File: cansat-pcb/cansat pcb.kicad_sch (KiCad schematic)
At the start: 19 parts, among them J1 Conn_01x03_Pin, J2 Conn_01x03_Pin, J3 Conn_01x03_Pin, Q1 2N3904, Q2 AO3400A, SW1 SW_DPDT_x2, U3 MPU6050

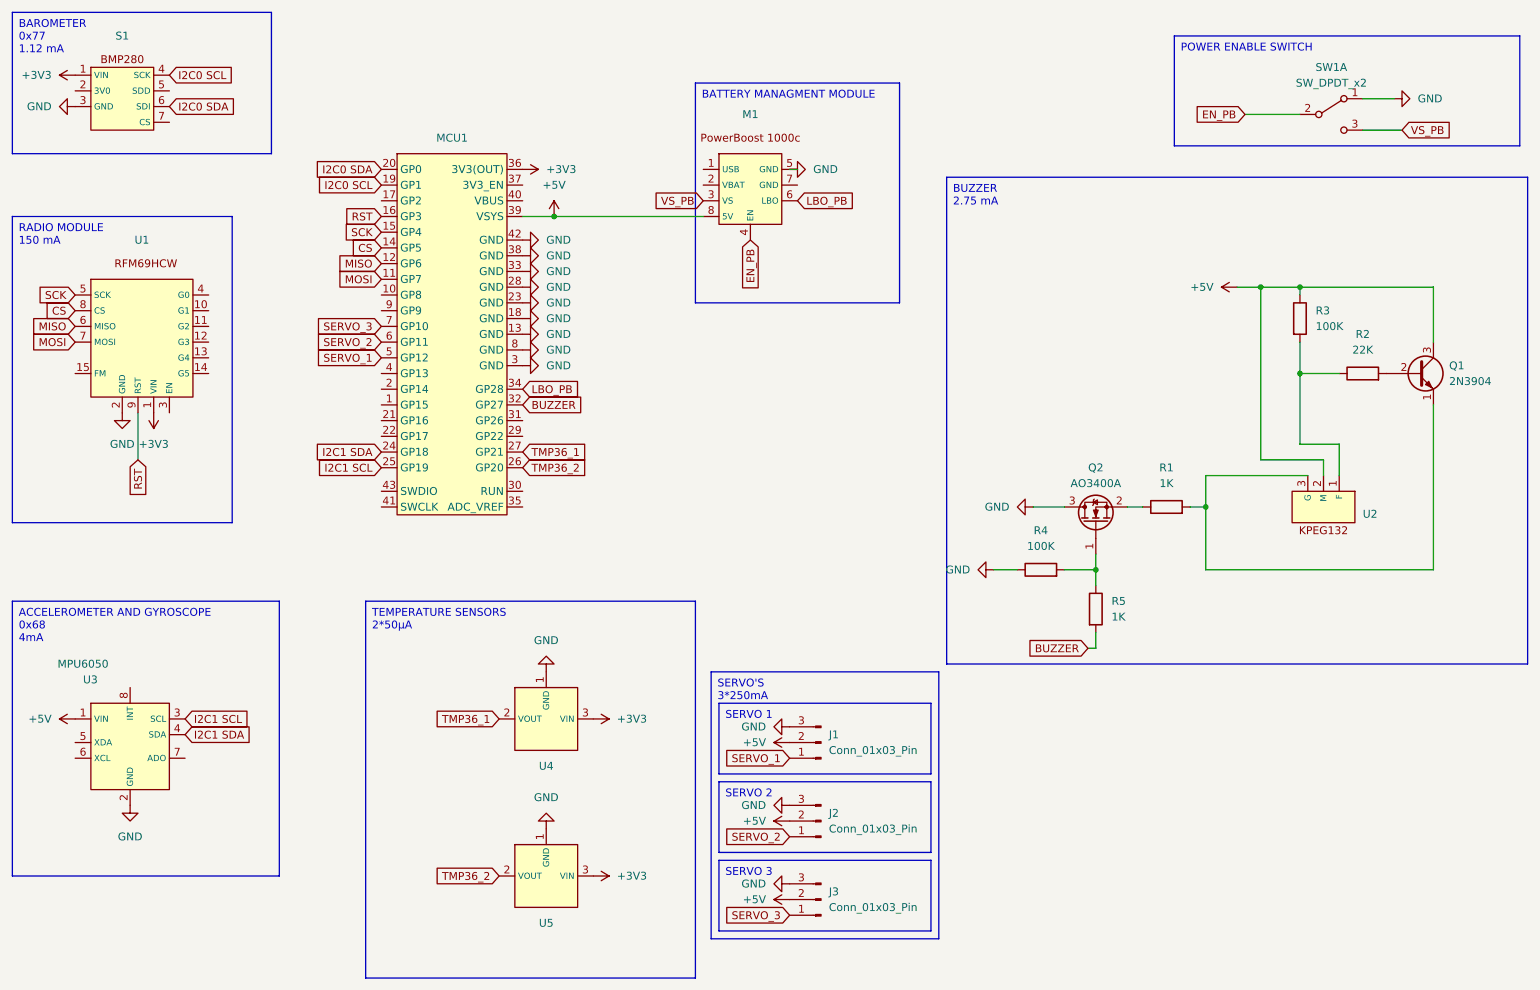
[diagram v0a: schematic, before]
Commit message: created MARKDOWN.md
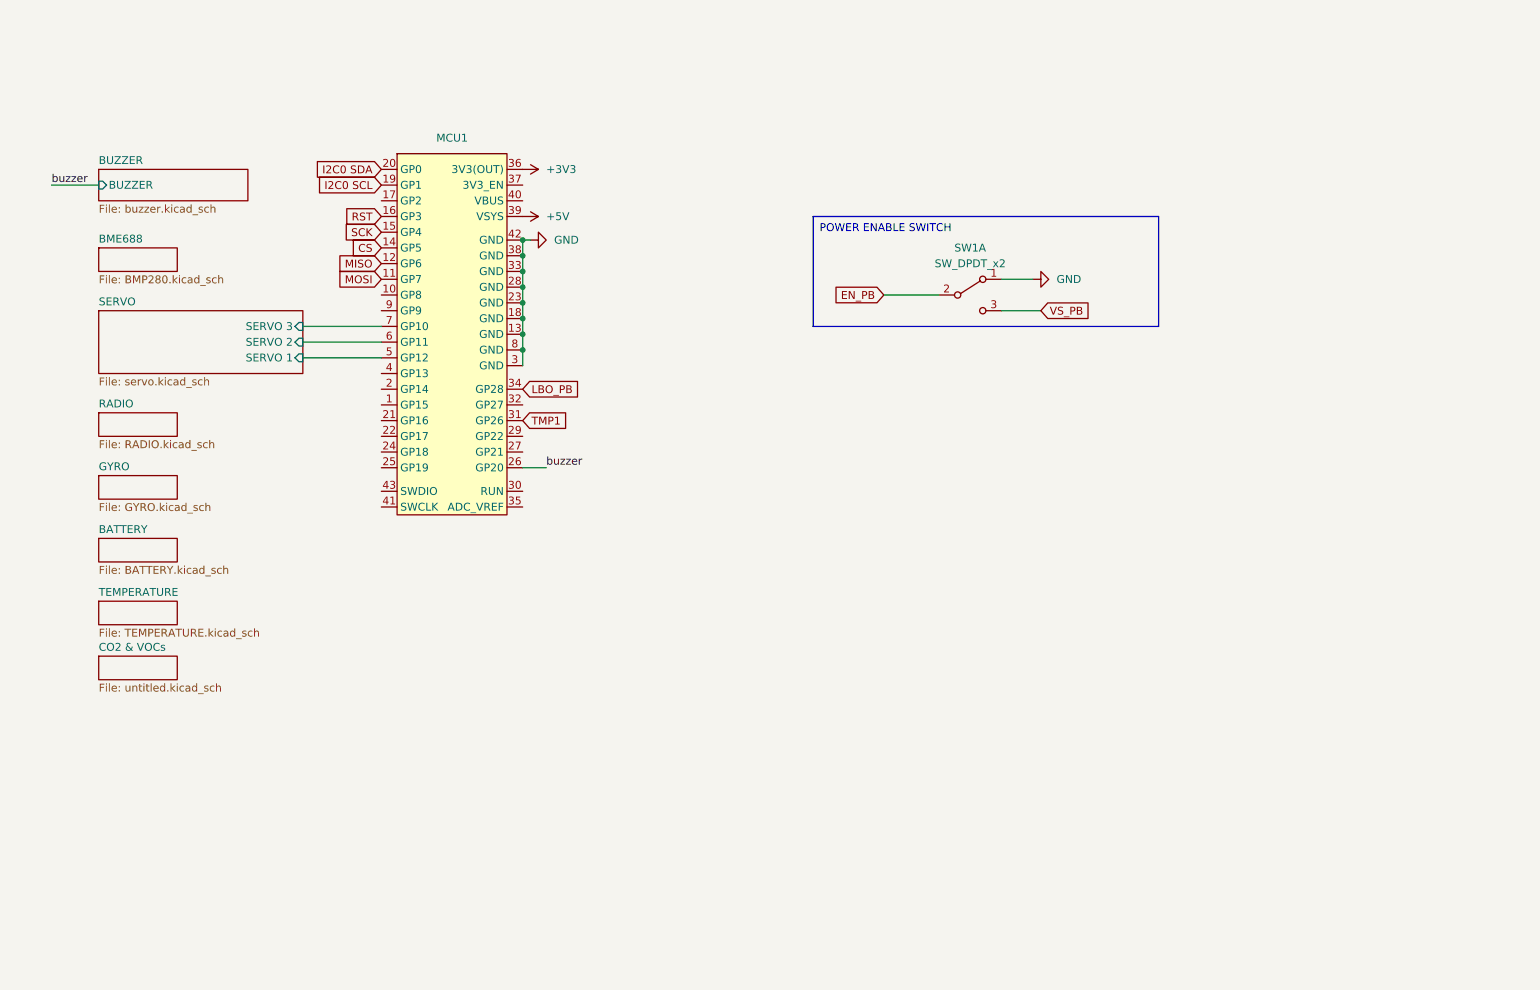
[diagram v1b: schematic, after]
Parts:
- removed J1, J2, J3: Conn_01x03_Pin, Connector_PinHeader_1.00mm:PinHeader_1x03_P1.00mm_Vertical, symbol Connector:Conn_01x03_Pin
- removed M1: ~, CanSat:PowerBoost, symbol CanSat:adafruit_PowerBoost_1000c
- removed Q1: 2N3904, Package_TO_SOT_THT:TO-92_Inline, symbol Transistor_BJT:2N3904
- removed Q2: AO3400A, Package_TO_SOT_SMD:SOT-23, symbol Transistor_FET:AO3400A
- removed R1, R5: 1K, Resistor_SMD:R_0805_2012Metric_Pad1.20x1.40mm_HandSolder, symbol Device:R
- removed R2: 22K, Resistor_SMD:R_0805_2012Metric_Pad1.20x1.40mm_HandSolder, symbol Device:R
- removed R3, R4: 100K, Resistor_SMD:R_0805_2012Metric_Pad1.20x1.40mm_HandSolder, symbol Device:R
- removed S1: ~, CanSat:BMP280, symbol CanSat:BMP280
- removed U1: ~, CanSat:RFM69HCW, symbol CanSat:RFM69HCW
- removed U2: ~, CanSat:KPEG132, symbol CanSat:KPEG132
- removed U3: MPU6050, CanSat:MPU6050, symbol CanSat:MPU6050
- removed U4, U5: ~, Package_TO_SOT_THT:TO-92L_Inline, symbol CanSat:TMP36
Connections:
- net TMP1: now reaches MCU1.31 (GP26)
- net BUZZER: no longer names the net of MCU1.32 (GP27)
- net I2C1 SCL: no longer names the net of MCU1.25 (GP19)
- net I2C1 SDA: no longer names the net of MCU1.24 (GP18)
- net SERVO_1 renamed SERVO/SERVO 1
- net SERVO_2 renamed SERVO/SERVO 2
- net SERVO_3 renamed SERVO/SERVO 3
- net TMP36_1: no longer names the net of MCU1.27 (GP21)
- net TMP36_2 renamed buzzer
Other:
- added sheet BATTERY (BATTERY.kicad_sch)
- added sheet BME688 (BMP280.kicad_sch)
- added sheet BUZZER (buzzer.kicad_sch)
- added sheet CO2 & VOCs (untitled.kicad_sch)
- added sheet GYRO (GYRO.kicad_sch)
- added sheet RADIO (RADIO.kicad_sch)
- added sheet SERVO (servo.kicad_sch)
- added sheet TEMPERATURE (TEMPERATURE.kicad_sch)
- moved on the sheet: SW1A
